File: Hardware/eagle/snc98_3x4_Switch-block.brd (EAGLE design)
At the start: 56.4 x 83.2 mm, 67 parts

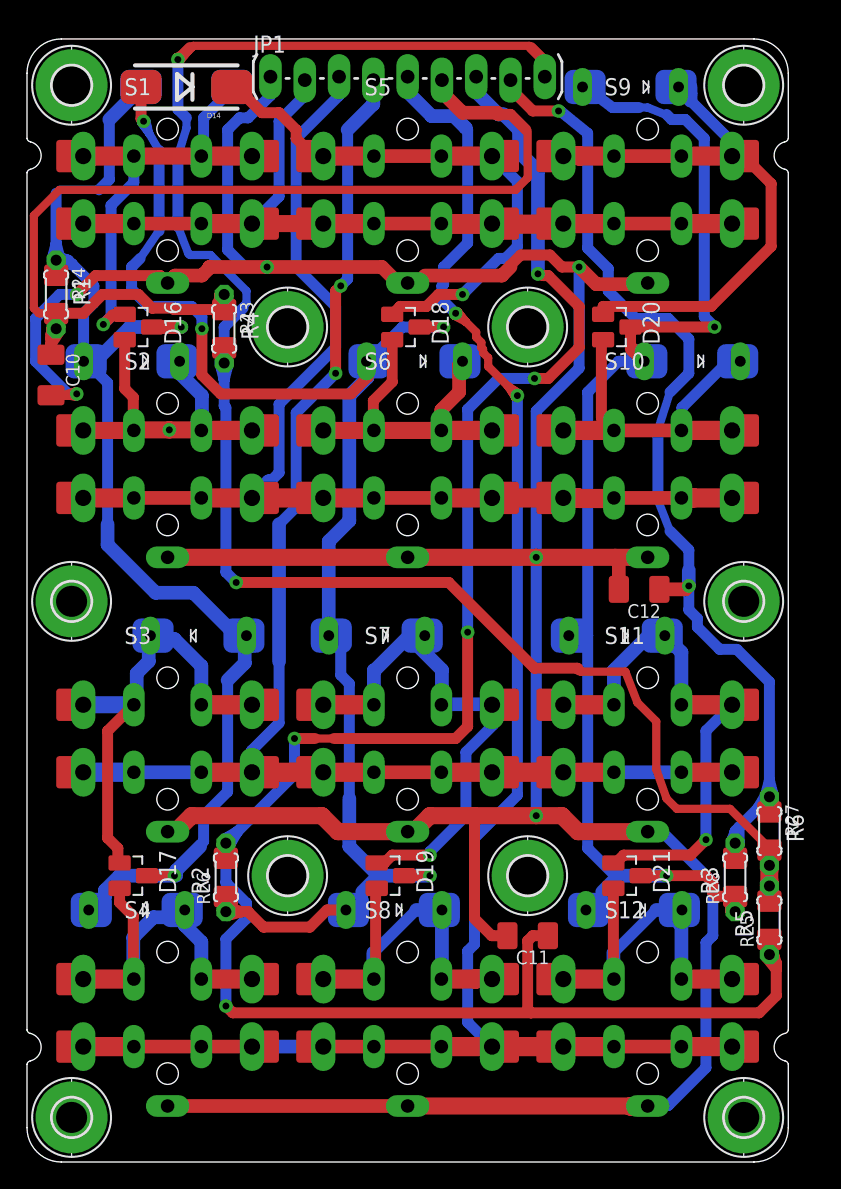
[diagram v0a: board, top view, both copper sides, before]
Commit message: Gerber file added
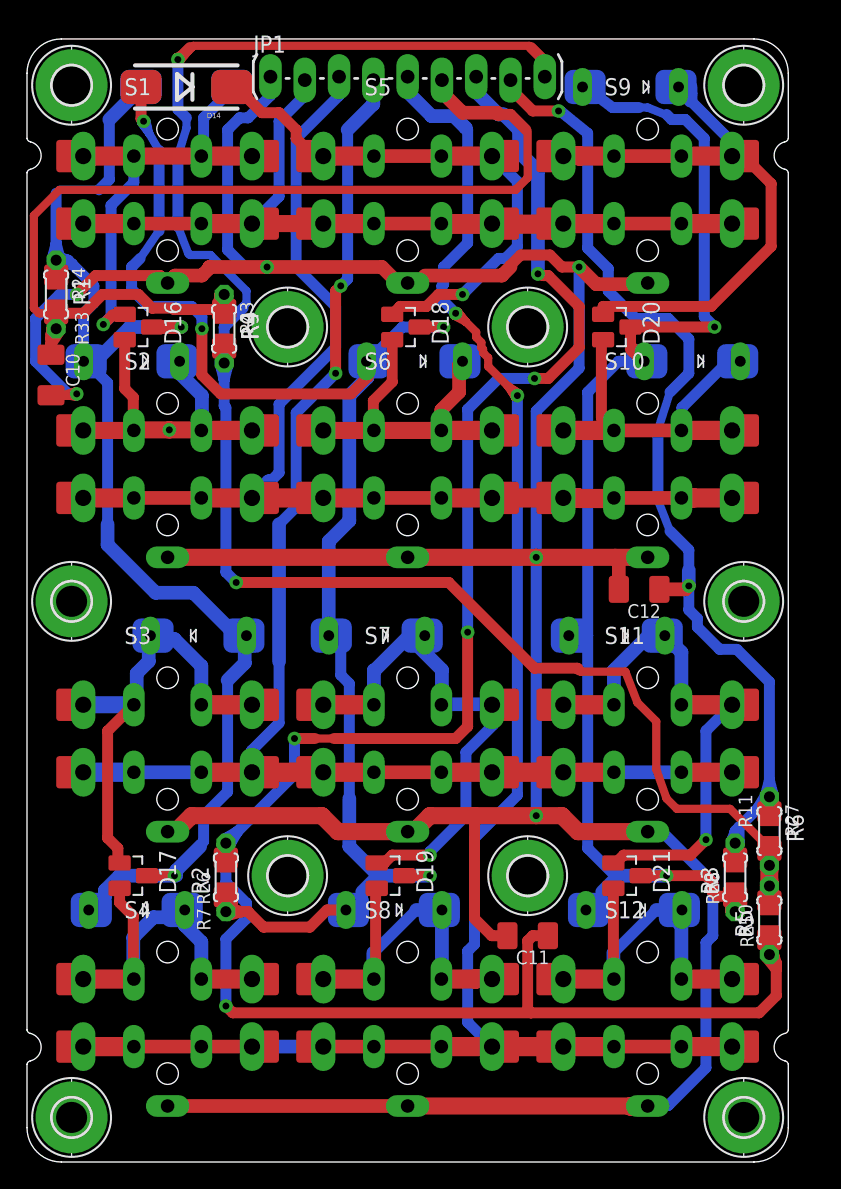
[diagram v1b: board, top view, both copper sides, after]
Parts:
- added R10, R11, R9: 27k, rcl:M0805
- added R33, R7, R8: 6k8, rcl:M0805
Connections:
- net A1: now also R33.2, R9.1
- net A2: now also R10.1, R7.2
- net A3: now also R11.1, R8.2
- net AREF: now also R10.2, R11.2, R9.2
- net A_1: now also R33.1
- net A_2: now also R7.1
- net A_3: now also R8.1
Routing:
- net AREF: track 172.8 -> 177.4 mm
- net A3: track 94.5 -> 97.5 mm
- net A2: track 167.4 -> 170.4 mm
- net A1: track 92.0 -> 95.0 mm
- net A_3: track 99.1 -> 100.6 mm
- net A_2: track 123.5 -> 125.0 mm
- net A_1: track 111.8 -> 113.3 mm
